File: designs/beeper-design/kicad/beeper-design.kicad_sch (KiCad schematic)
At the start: 0 parts

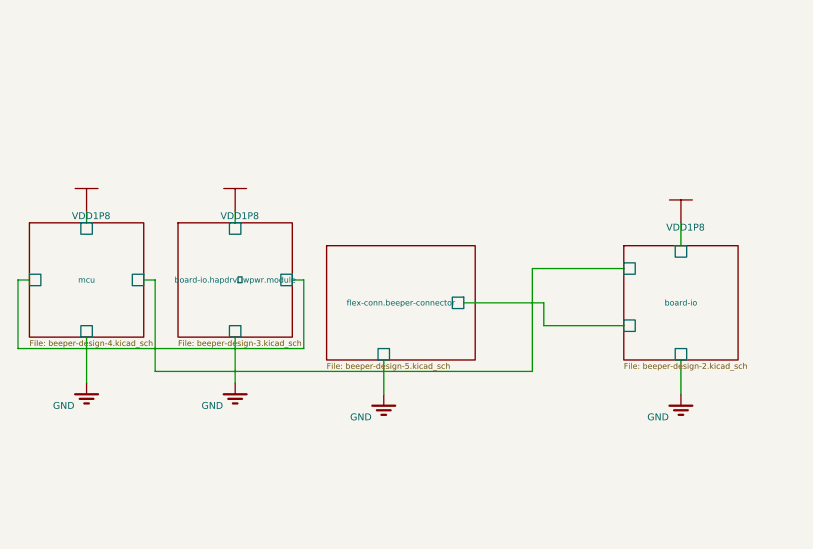
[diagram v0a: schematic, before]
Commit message: updated kicad export
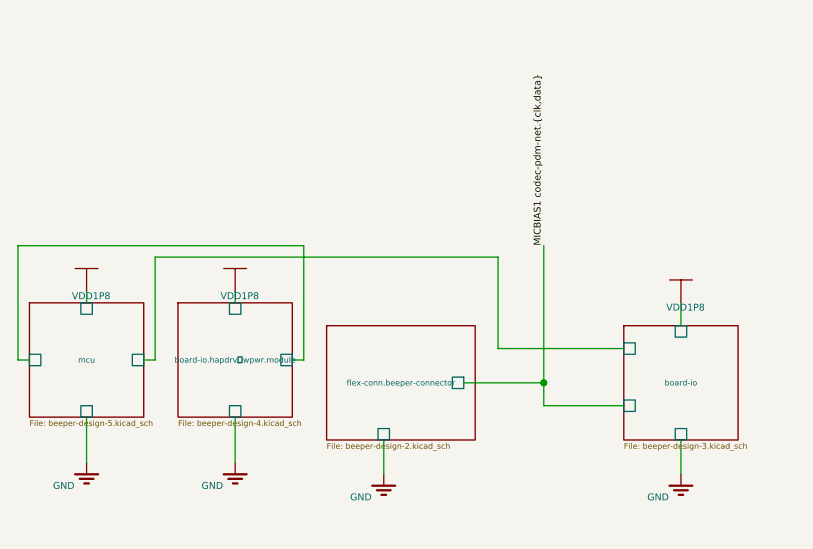
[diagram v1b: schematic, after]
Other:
- sheet board-io: file beeper-design-2.kicad_sch -> beeper-design-3.kicad_sch
- sheet board-io.hapdrv wpwr.module: file beeper-design-3.kicad_sch -> beeper-design-4.kicad_sch
- sheet flex-conn.beeper-connector: file beeper-design-5.kicad_sch -> beeper-design-2.kicad_sch
- sheet mcu: file beeper-design-4.kicad_sch -> beeper-design-5.kicad_sch

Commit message: exported yet again
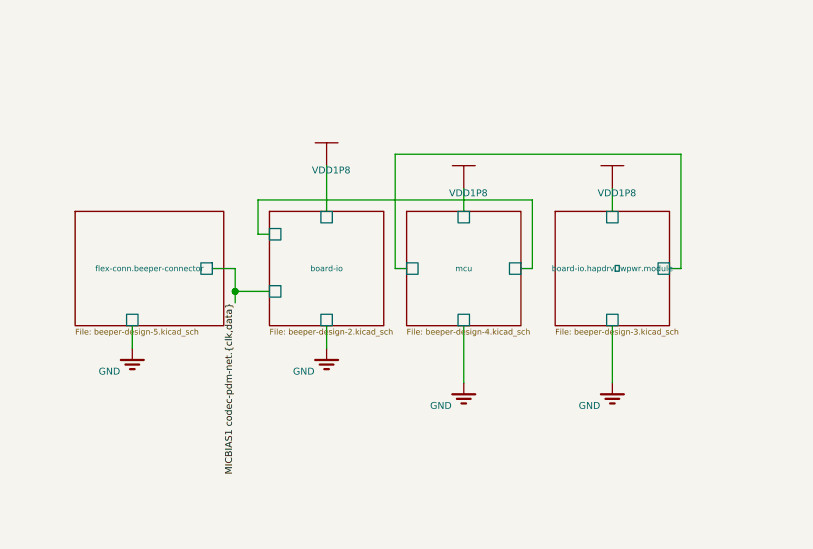
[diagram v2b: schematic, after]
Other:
- sheet board-io: file beeper-design-3.kicad_sch -> beeper-design-2.kicad_sch
- sheet board-io.hapdrv wpwr.module: file beeper-design-4.kicad_sch -> beeper-design-3.kicad_sch
- sheet flex-conn.beeper-connector: file beeper-design-2.kicad_sch -> beeper-design-5.kicad_sch
- sheet mcu: file beeper-design-5.kicad_sch -> beeper-design-4.kicad_sch

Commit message: exported yet again 2
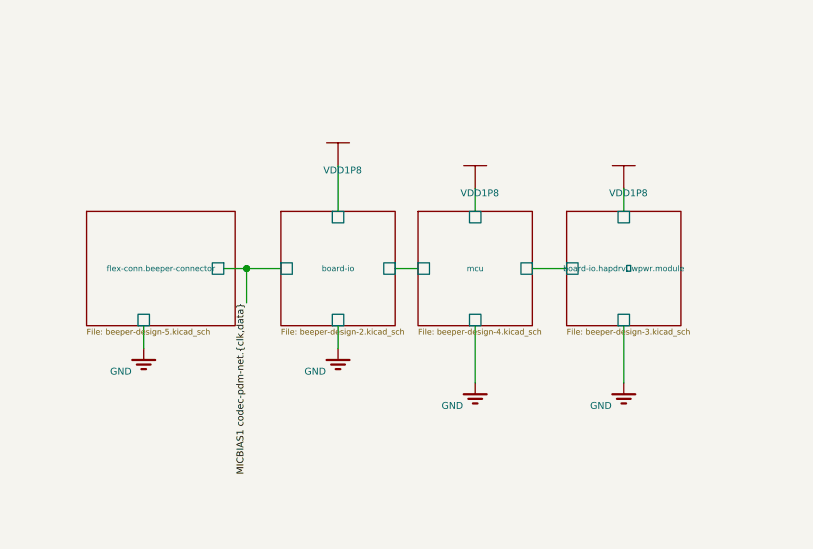
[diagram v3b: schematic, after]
